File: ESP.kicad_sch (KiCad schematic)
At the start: 37 parts, among them J5 B4B-ZRLFSN, P1 B6B-ZRLFSN, P2 B6B-ZRLFSN, P3 B6B-ZRLFSN, P4 S6B-ZRLFSN, P5 B6B-ZRLFSN, P6 B6B-ZRLFSN, U3 DRV8835DSSR, U4 RP2040, U5 DRV8835DSSR, U6 DRV8835DSSR, U7 W25X40CLSS, Y1 ABM8G-12.000MHZ-4Y-T3

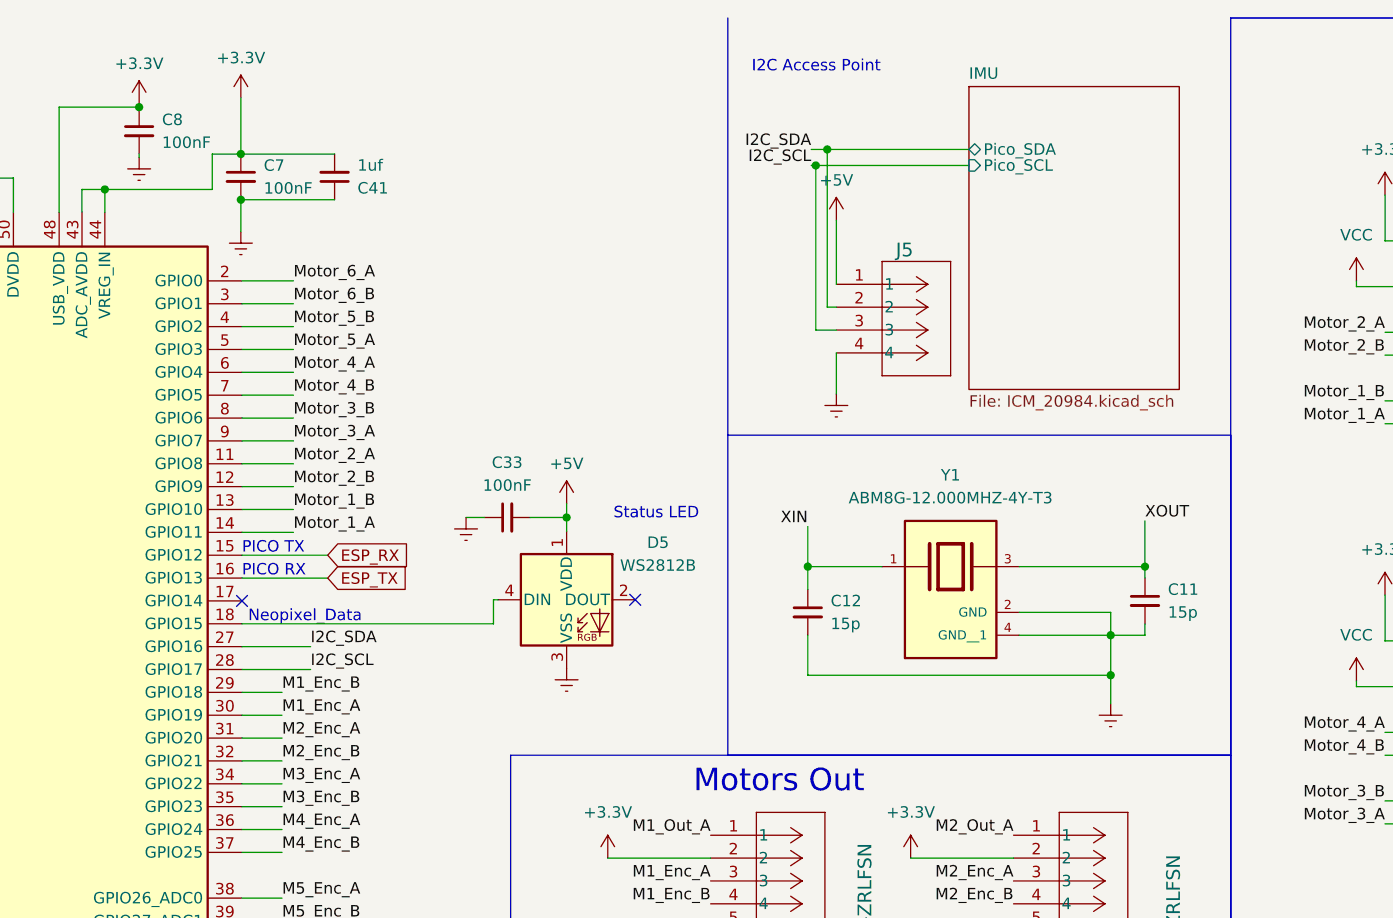
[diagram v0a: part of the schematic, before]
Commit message: Rev0.1
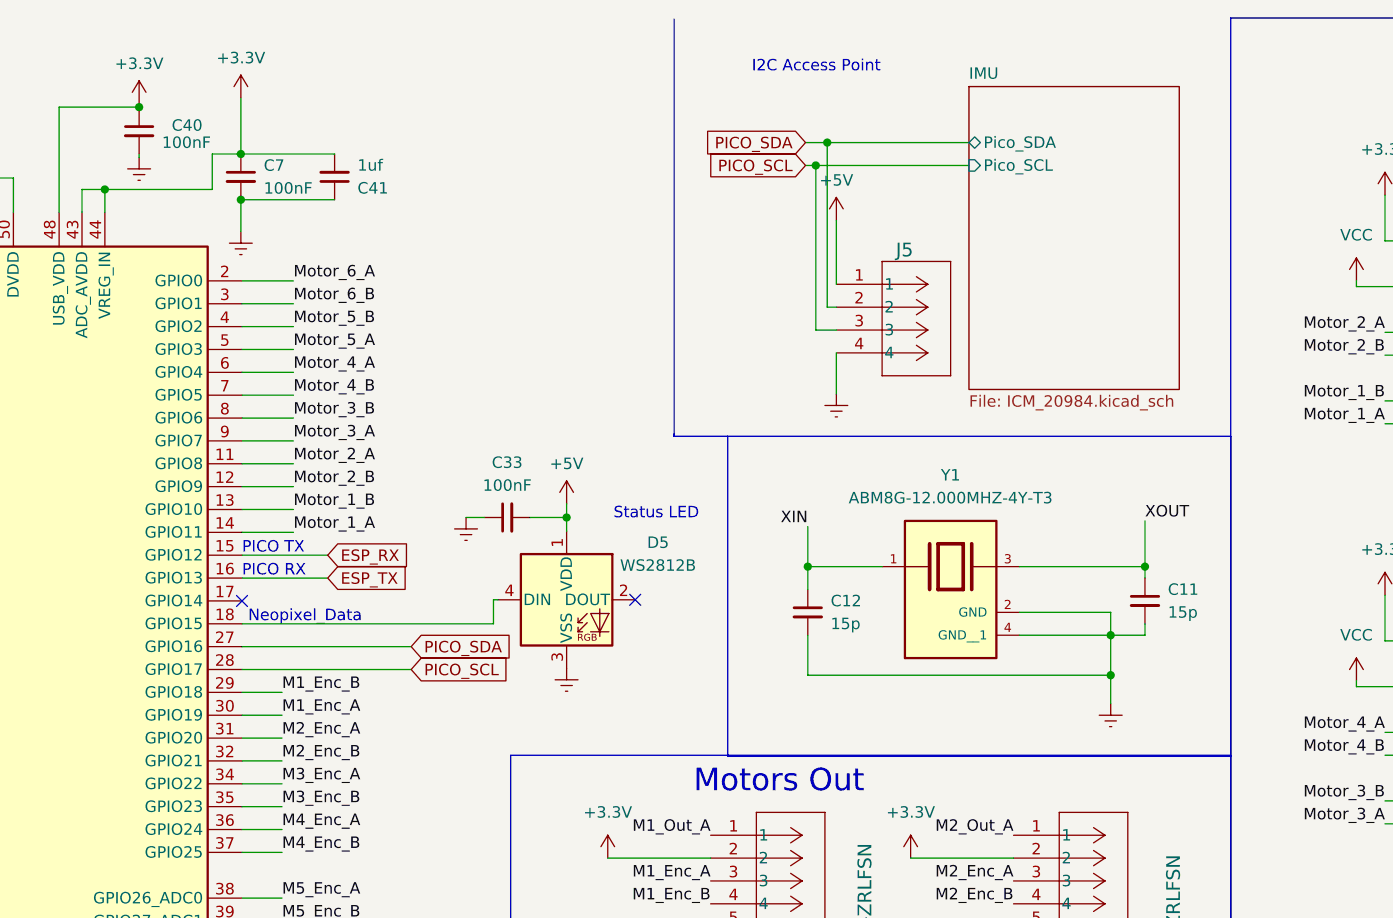
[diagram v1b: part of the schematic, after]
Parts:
- C8: Name (none) -> C40
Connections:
- net I2C_SCL renamed PICO_SCL
- net I2C_SDA renamed PICO_SDA
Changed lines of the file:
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@@
   (junction (at 266.7 106.68) (diameter 0) (color 0 0 0 0)
   )
-  (junction (at 161.544 26.67) (diameter 0) (color 0 0 0 0)
+  (junction (at 161.544 25.908) (diameter 0) (color 0 0 0 0)
   )
   (junction (at 59.563 29.845) (diameter 0) (color 0 0 0 0)
@@
     (stroke (width 0) (type default))
   )
-  (wire (pts (xy 159.766 28.448) (xy 160.274 28.448))
+  (wire (pts (xy 159.131 28.448) (xy 160.274 28.448))
+    (stroke (width 0) (type default))
+  )
+  (polyline (pts (xy 144.526 58.293) (xy 144.526 58.547))
     (stroke (width 0) (type default))
   )
@@
     (stroke (width 0) (type default))
   )
+  (polyline (pts (xy 150.495 58.547) (xy 144.526 58.547))
+    (stroke (width 0) (type default))
+  )
   (wire (pts (xy 140.335 179.705) (xy 146.685 179.705))
     (stroke (width 0) (type default))
@@
     (stroke (width 0) (type default))
   )
-  (wire (pts (xy 159.766 26.67) (xy 161.544 26.67))
+  (wire (pts (xy 159.131 25.908) (xy 161.544 25.908))
     (stroke (width 0) (type default))
   )
@@
     (stroke (width 0) (type default))
   )
-  (wire (pts (xy 104.14 81.915) (xy 96.52 81.915))
+  (wire (pts (xy 115.316 81.915) (xy 96.52 81.915))
     (stroke (width 0) (type default))
   )
@@
     (stroke (width 0) (type default))
   )
-  (polyline (pts (xy 150.495 12.065) (xy 150.495 58.42))
+  (polyline (pts (xy 144.526 12.192) (xy 144.526 58.547))
     (stroke (width 0) (type default))
   )
-  (wire (pts (xy 161.544 26.67) (xy 161.544 44.196))
+  (wire (pts (xy 161.544 25.908) (xy 161.544 44.196))
     (stroke (width 0) (type default))
   )
@@
     (stroke (width 0) (type default))
   )
-  (wire (pts (xy 161.544 26.67) (xy 177.292 26.67))
+  (wire (pts (xy 161.544 25.908) (xy 177.292 25.908))
     (stroke (width 0) (type default))
   )
@@
     (stroke (width 0) (type default))
   )
-  (wire (pts (xy 104.14 84.455) (xy 96.52 84.455))
+  (wire (pts (xy 115.316 84.455) (xy 96.52 84.455))
     (stroke (width 0) (type default))
   )
@@
     (fill (type none))
   )
-  (rectangle (start 150.495 58.42) (end 206.375 93.98)
+  (rectangle (start 150.495 58.547) (end 206.375 94.107)
     (stroke (width 0) (type default))
     (fill (type none))
@@
     (effects (font (size 1.27 1.27)) (justify left bottom))
   )
-  (label "I2C_SCL" (at 104.14 84.455 0) (fields_autoplaced)
-    (effects (font (size 1.27 1.27)) (justify left bottom))
-  )
   (label "M6_Out_A" (at 271.78 125.73 0) (fields_autoplaced)
     (effects (font (size 1.27 1.27)) (justify left bottom))
@@
     (effects (font (size 1.27 1.27)) (justify left bottom))
   )
-  (label "I2C_SDA" (at 104.14 81.915 0) (fields_autoplaced)
-    (effects (font (size 1.27 1.27)) (justify left bottom))
-  )
   (label "M4_Out_A" (at 270.51 81.28 0) (fields_autoplaced)
     (effects (font (size 1.27 1.27)) (justify left bottom))
@@
     (effects (font (size 1.27 1.27)) (justify right bottom))
   )
-  (label "I2C_SDA" (at 159.766 26.67 180) (fields_autoplaced)
-    (effects (font (size 1.27 1.27)) (justify right bottom))
-  )
   (label "M2_Out_A" (at 182.245 102.87 180) (fields_autoplaced)
     (effects (font (size 1.27 1.27)) (justify right bottom))
@@
     (effects (font (size 1.27 1.27)) (justify right bottom))
   )
-  (label "I2C_SCL" (at 159.766 28.448 180) (fields_autoplaced)
-    (effects (font (size 1.27 1.27)) (justify right bottom))
-  )
   (label "XIN" (at 33.655 94.615 180) (fields_autoplaced)
     (effects (font (size 1.27 1.27)) (justify right bottom))
@@
     )
   )
+  (global_label "PICO_SDA" (shape input) (at 159.131 25.908 180) (fields_autoplaced)
+    (effects (font (size 1.27 1.27)) (justify right))
+    (property "Intersheetrefs" "${INTERSHEET_REFS}" (at 147.1348 25.908 0)
+      (effects (font (size 1.27 1.27)) (justify right) hide)
+    )
+  )
+  (global_label "PICO_SDA" (shape input) (at 115.316 81.915 0) (fields_autoplaced)
+    (effects (font (size 1.27 1.27)) (justify left))
+    (property "Intersheetrefs" "${INTERSHEET_REFS}" (at 127.3122 81.915 0)
+      (effects (font (size 1.27 1.27)) (justify left) hide)
+    )
+  )
   (global_label "ESP_TX" (shape input) (at 106.045 74.295 0) (fields_autoplaced)
     (effects (font (size 1.27 1.27)) (justify left))
@@
     )
   )
+  (global_label "PICO_SCL" (shape input) (at 159.131 28.448 180) (fields_autoplaced)
+    (effects (font (size 1.27 1.27)) (justify right))
+    (property "Intersheetrefs" "${INTERSHEET_REFS}" (at 147.1953 28.448 0)
+      (effects (font (size 1.27 1.27)) (justify right) hide)
+    )
+  )
+  (global_label "PICO_SCL" (shape input) (at 115.316 84.455 0) (fields_autoplaced)
+    (effects (font (size 1.27 1.27)) (justify left))
+    (property "Intersheetrefs" "${INTERSHEET_REFS}" (at 127.2517 84.455 0)
+      (effects (font (size 1.27 1.27)) (justify left) hide)
+    )
+  )
   (hierarchical_label "Pico_PU" (shape input) (at 30.48 41.275 180) (fields_autoplaced)
     (effects (font (size 1.27 1.27)) (justify right))
@@
   )
   (symbol (lib_id "Device:C_Small") (at 85.09 24.638 0) (unit 1)
-    (in_bom yes) (on_board yes) (dnp no) (fields_autoplaced)
+    (in_bom yes) (on_board no) (dnp no)
     (property "Reference" "C8" (at 87.63 23.3743 0)
-      (effects (font (size 1.27 1.27)) (justify left))
+      (effects (font (size 1.27 1.27)) (justify left) hide)
     )
     (property "Value" "100nF" (at 87.63 25.9143 0)
@@
       (effects (font (size 1.27 1.27)) hide)
     )
+    (property "Sim.Enable" "0" (at 85.09 24.638 0)
+      (effects (font (size 1.27 1.27)) hide)
+    )
+    (property "Name" "C40" (at 90.424 24.003 0)
+      (effects (font (size 1.27 1.27)))
+    )
     (pin "1")
     (pin "2")
@@
       (effects (font (size 1.27 1.27)) (justify left top))
     )
-    (pin "Pico_SDA" bidirectional (at 177.292 26.67 180)
+    (pin "Pico_SDA" bidirectional (at 177.292 25.908 180)
       (effects (font (size 1.27 1.27)) (justify left))
     )

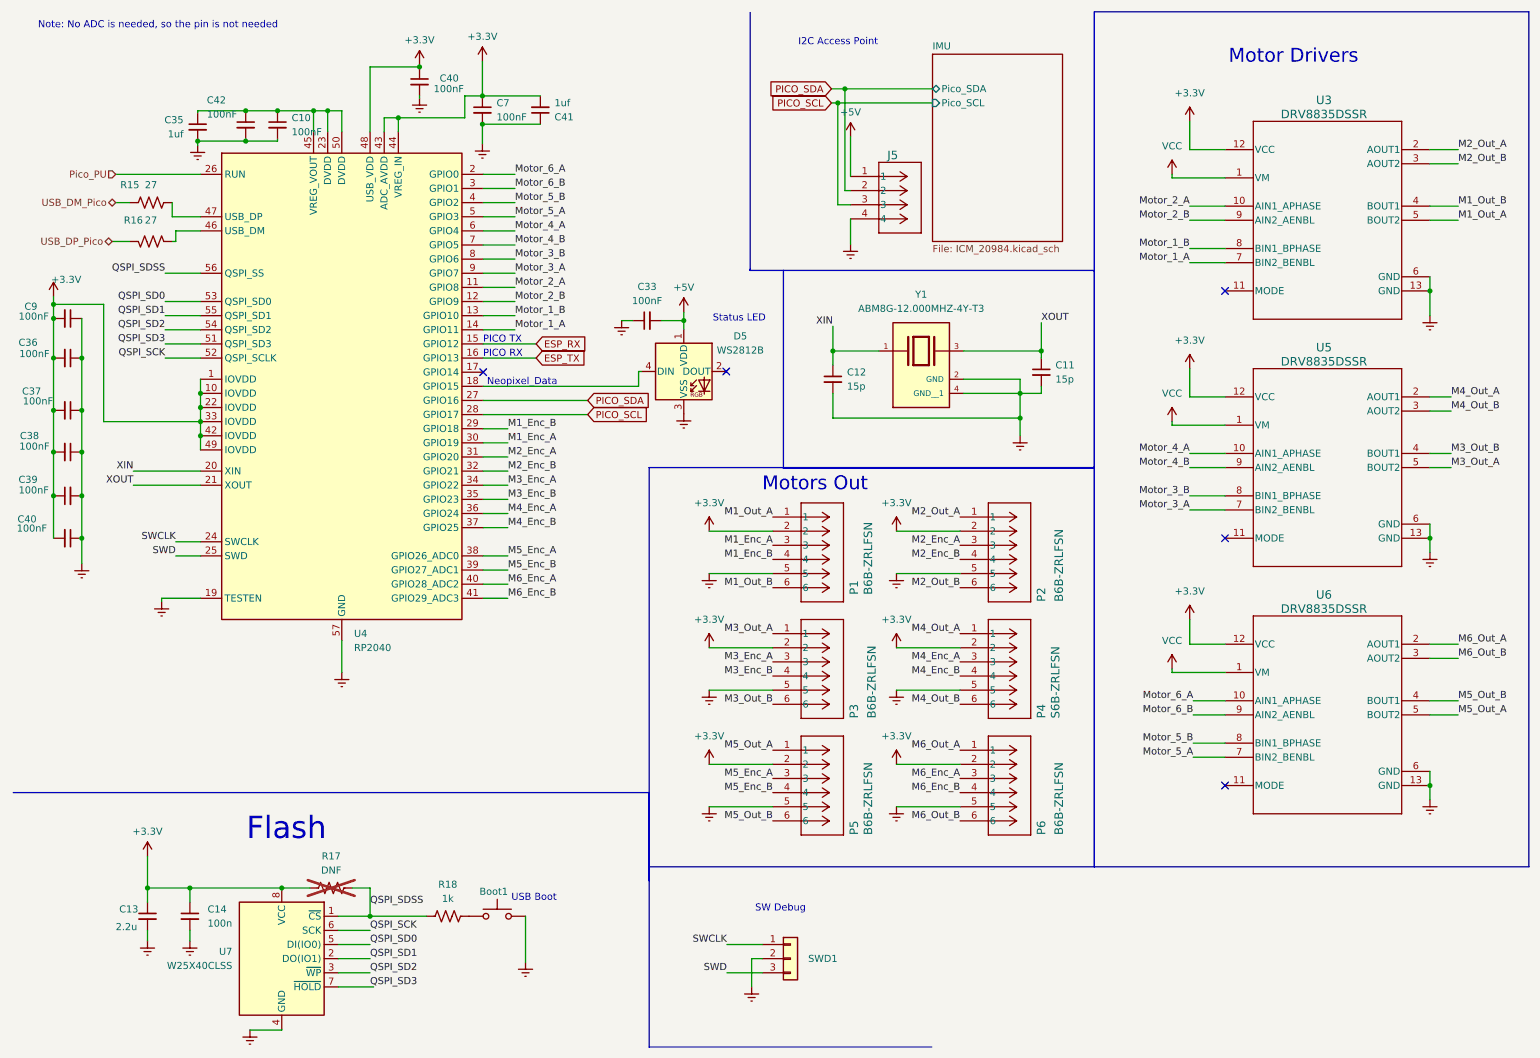
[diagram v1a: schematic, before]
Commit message: clean up Rev
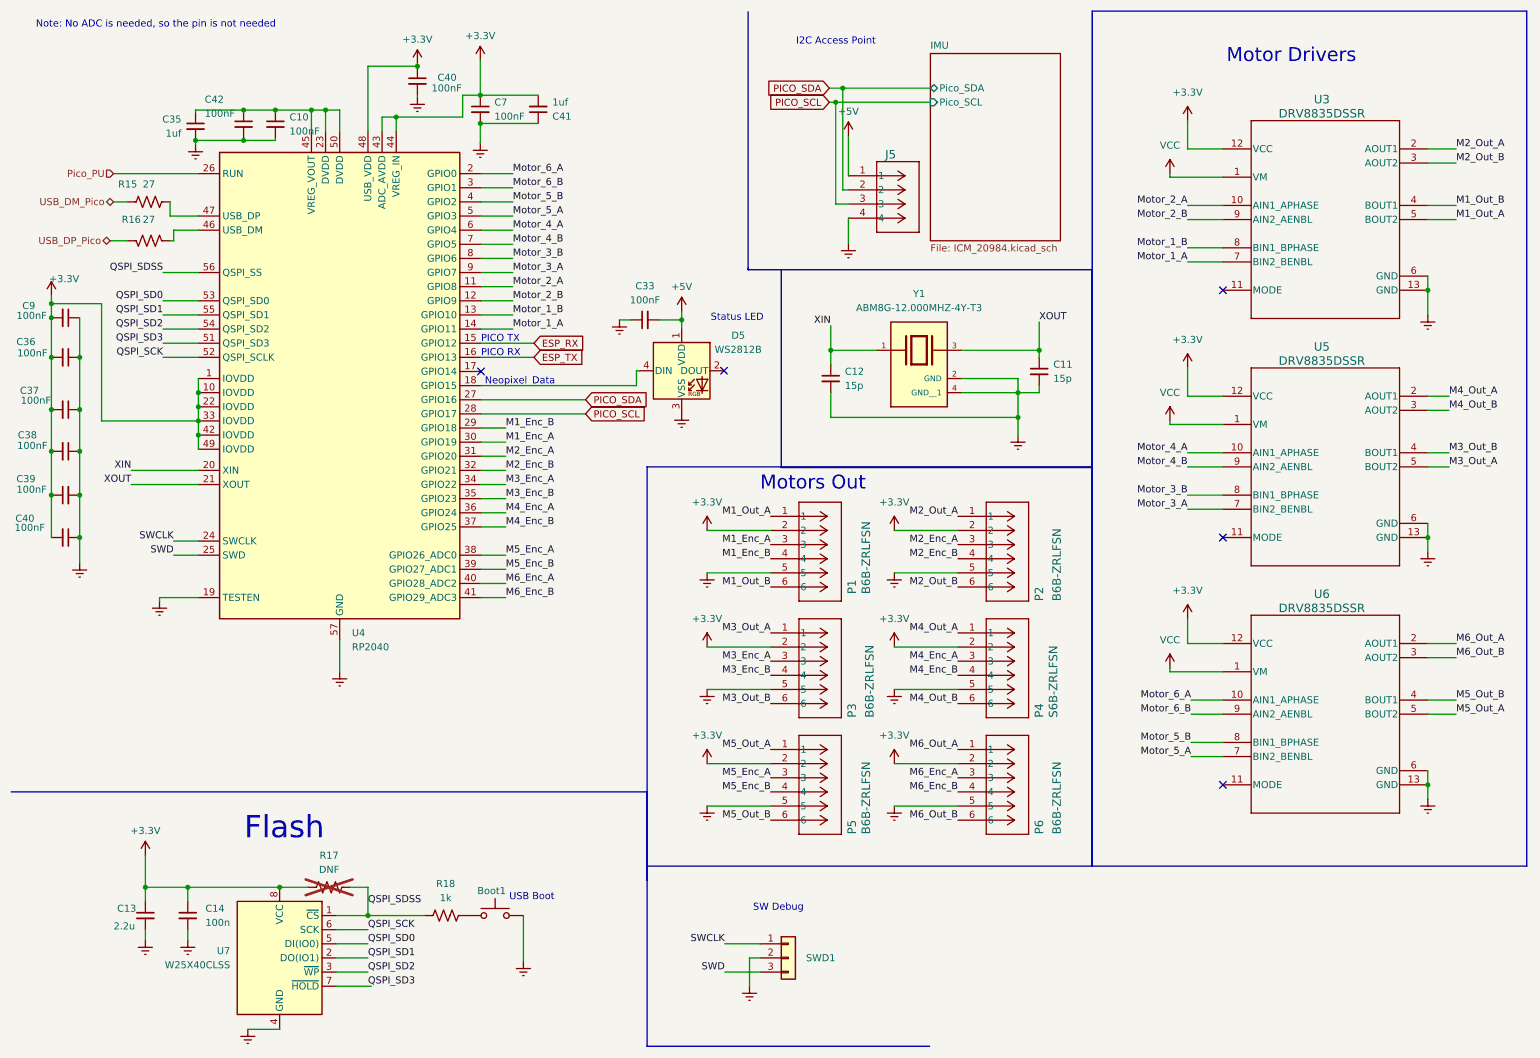
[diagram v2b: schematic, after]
